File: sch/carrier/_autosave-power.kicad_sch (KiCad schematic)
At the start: 33 parts, among them U3 MP2636GR-P

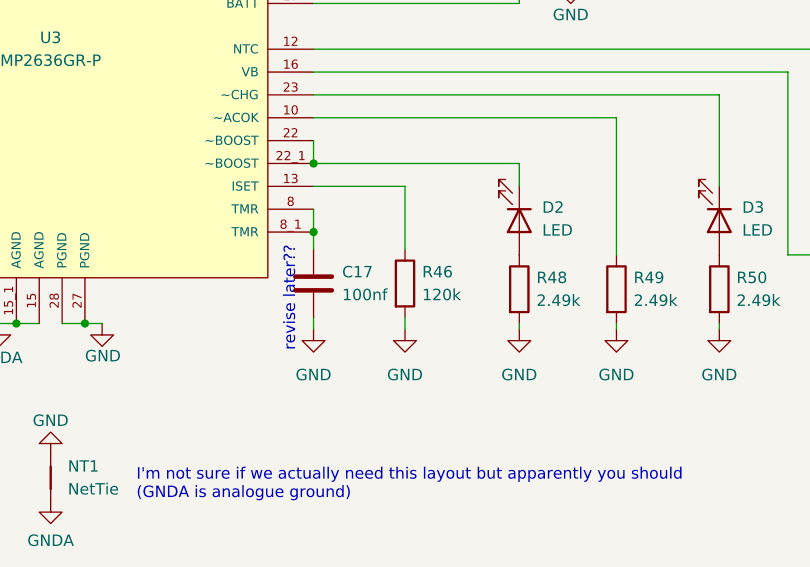
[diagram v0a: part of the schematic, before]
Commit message: aa
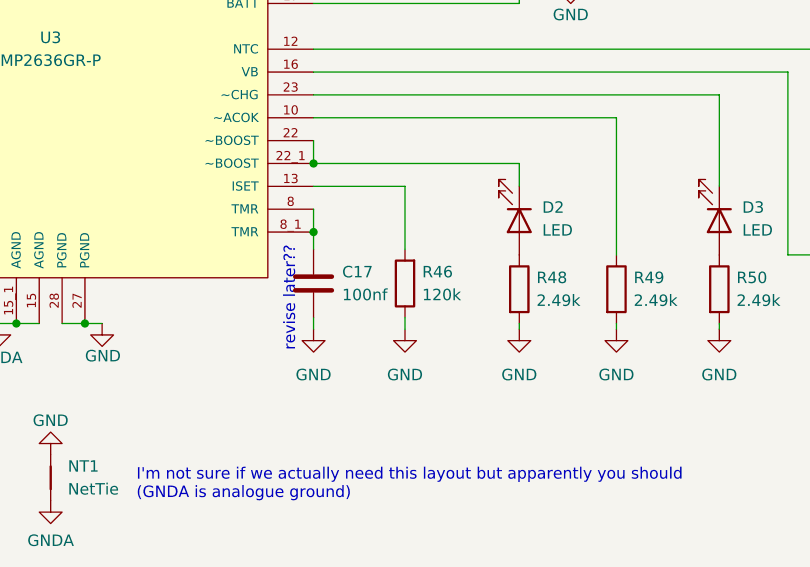
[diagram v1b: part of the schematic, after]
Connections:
- net GND: now also R46.1; no longer R46.2
- net at U3.13 (ISET): now also R46.2; no longer R46.1
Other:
- moved on the sheet: R46
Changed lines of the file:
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@@
     (pin "2")
   )
-  (symbol (lib_id "Device:R") (at 186.055 97.155 0) (unit 1)
+  (symbol (lib_id "Device:R") (at 186.055 97.155 180) (unit 1)
     (in_bom yes) (on_board yes) (fields_autoplaced)
     (property "Reference" "R46" (id 0) (at 187.96 95.8849 0)
-      (effects (font (size 1.27 1.27)) (justify left))
+      (effects (font (size 1.27 1.27)) (justify right))
     )
     (property "Value" "120k" (id 1) (at 187.96 98.4249 0)
-      (effects (font (size 1.27 1.27)) (justify left))
+      (effects (font (size 1.27 1.27)) (justify right))
     )
-    (property "Footprint" "Resistor_SMD:R_0402_1005Metric_Pad0.72x0.64mm_HandSolder" (id 2) (at 184.277 97.155 90)
+    (property "Footprint" "Resistor_SMD:R_0402_1005Metric_Pad0.72x0.64mm_HandSolder" (id 2) (at 187.833 97.155 90)
       (effects (font (size 1.27 1.27)) hide)
     )
@@
   )
   (symbol (lib_id "Device:R") (at 252.73 90.17 0) (unit 1)
-    (in_bom yes) (on_board yes) (fields_autoplaced)
+    (in_bom yes) (on_board yes)
     (property "Reference" "R53" (id 0) (at 254.635 88.8999 0)
       (effects (font (size 1.27 1.27)) (justify left))
